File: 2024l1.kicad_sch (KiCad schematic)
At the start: 58 parts, among them IC1 SN74LVC2G04DBVTG4, IC2 SN74LVC2G04DBVTG4, M1 VNH5050A-E, M1C1 680u, M1C2 33n, M1R1 3K3, M1R2 3K3, M1R3 1K, M1R4 1K, M1R5 1K, M1R6 1K, M1R7 1K, M1R8 10K, M1R9 1K5, M1_CONN XT30, M2 VNH5050A-E, M2C2 33n, M2C2 680u, M2R1 3K3, M2R2 3K3, M2R3 1K, M2R4 1K, M2R5 1K, M2R6 1K, M2R7 1K, M2R8 10K, M2R9 1K5, M2_CONN XT30, M3 VNH5050A-E, M3C1 680u, M3C2 33n, M3R1 3K3, M3R2 3K3, M3R3 1K, M3R4 1K, M3R5 1K, M3R6 1K, M3R7 1K, M3R8 10K, M3R9 1K5, M3_CONN XT30, M4 VNH5050A-E, M4C1 680u, M4C2 33n, M4R1 3K3, M4R2 3K3, M4R3 1K, M4R4 1K, M4R5 1K, M4R6 1K, M4R7 1K, M4R8 10K, M4R9 1K5, M4_CONN XT30

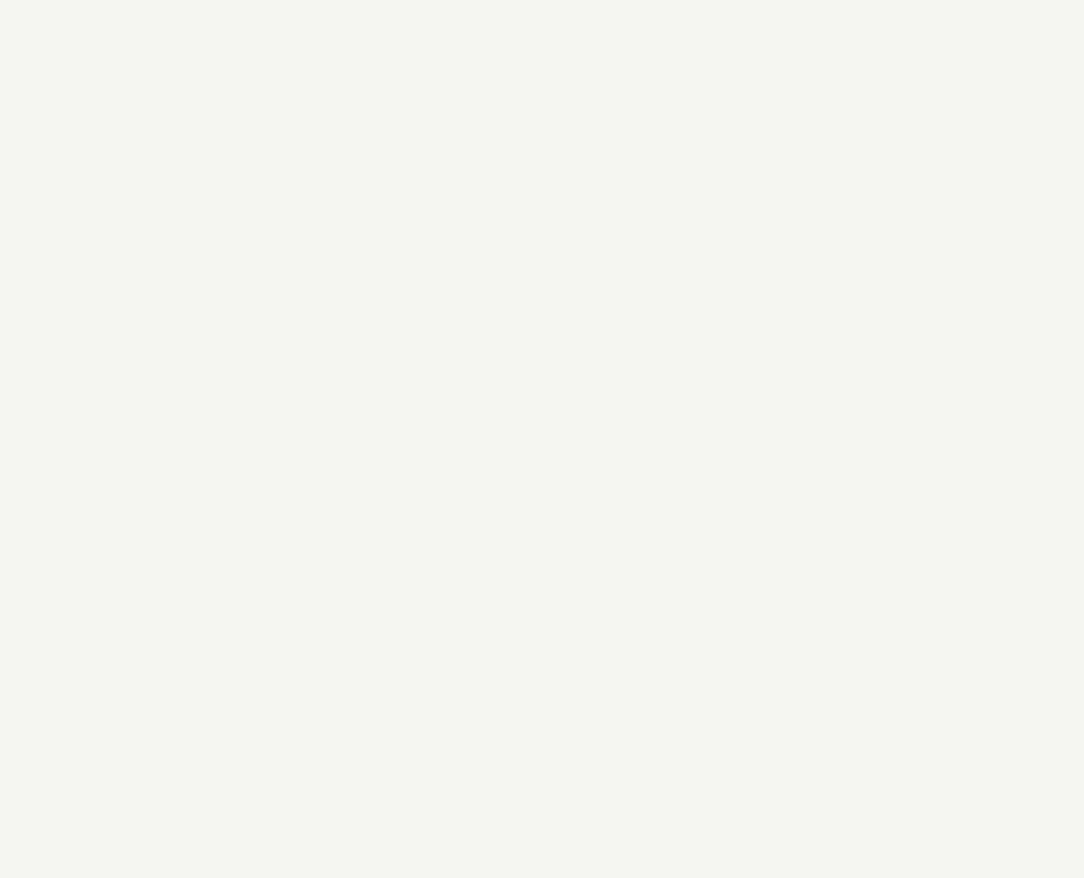
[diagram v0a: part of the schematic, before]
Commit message: buck conv
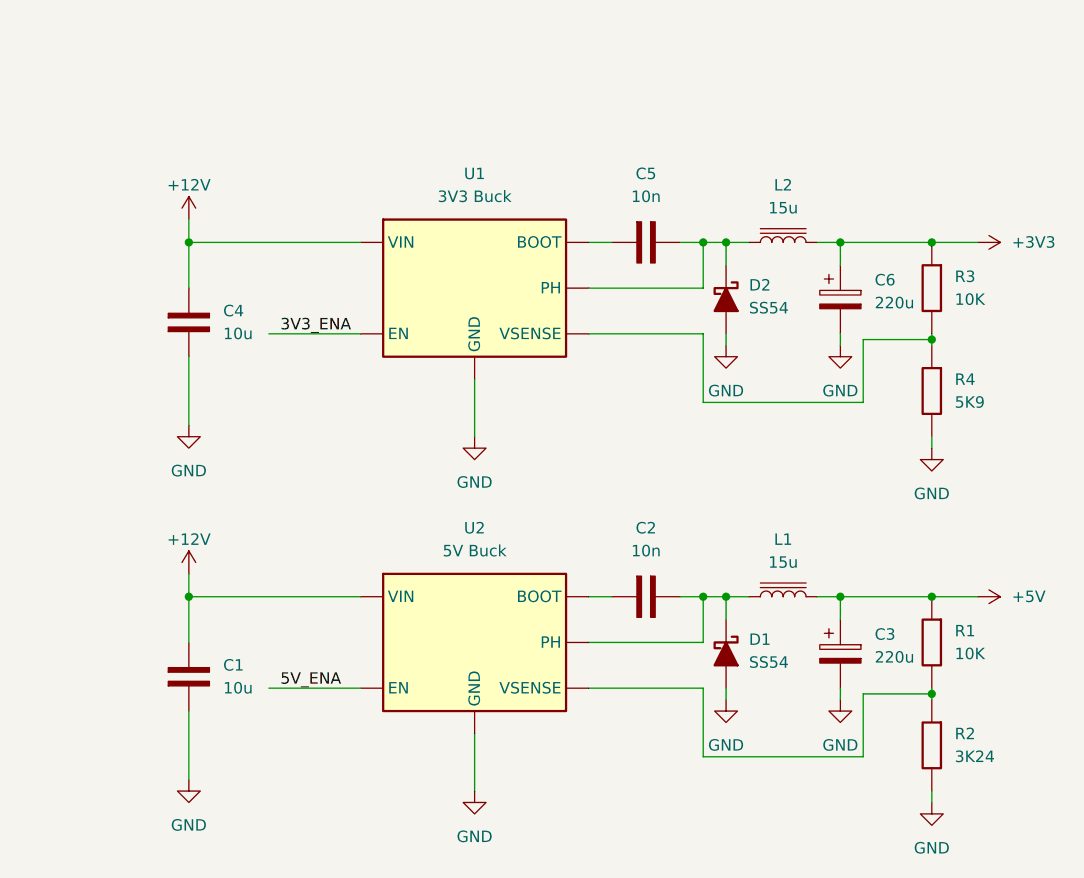
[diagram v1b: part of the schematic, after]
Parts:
- added C1, C4: 10u, symbol vincent:C
- added C2, C5: 10n, symbol vincent:C
- added C3, C6: 220u, symbol vincent:C_Polarized
- added D1, D2: SS54, symbol vincent:D_Schotty
- added L1, L2: 15u, symbol vincent:L_Iron
- added R1, R3: 10K, symbol vincent:R
- added R2: 3K24, symbol vincent:R
- added R4: 5K9, symbol vincent:R
- added U1: 3V3 Buck, symbol vincent:TPS5430
- added U2: 5V Buck, symbol vincent:TPS5430
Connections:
- net +3V3: now also C6.1, L2.2, R3.2
- net +5V: now also C3.1, L1.2, R1.2
- net GND: now also C1.1, C3.2, C4.1, C6.2, D1.2, D2.2, R2.1, R4.1, U1.6,9 (GND), U2.6,9 (GND)
- new net: R1.1, R2.2, U2.4 (VSENSE)
- new net: C2.2, D1.1, L1.1, U2.8 (PH)
- new net: R3.1, R4.2, U1.4 (VSENSE)
- new net: C5.1, U1.1 (BOOT)
- new net: C5.2, D2.1, L2.1, U1.8 (PH)
- new net: C2.1, U2.1 (BOOT)
- new net +12V: C1.2, C4.2, U1.7 (VIN), U2.7 (VIN)
- new net 3V3_ENA: U1.5 (EN)
- new net 5V_ENA: U2.5 (EN)
